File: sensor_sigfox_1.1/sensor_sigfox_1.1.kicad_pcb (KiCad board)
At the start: 2 copper layers, 27.8 x 60.1 mm, 18 parts, among them IC1 WSSFM11R2DAT, J1 Battery, J2 Conn_01x07_Socket, J3 Conn_01x01_Female, J4 Antenna, U1 ATtiny826-X, U2 MLX90393, Y1 32.768 kHz

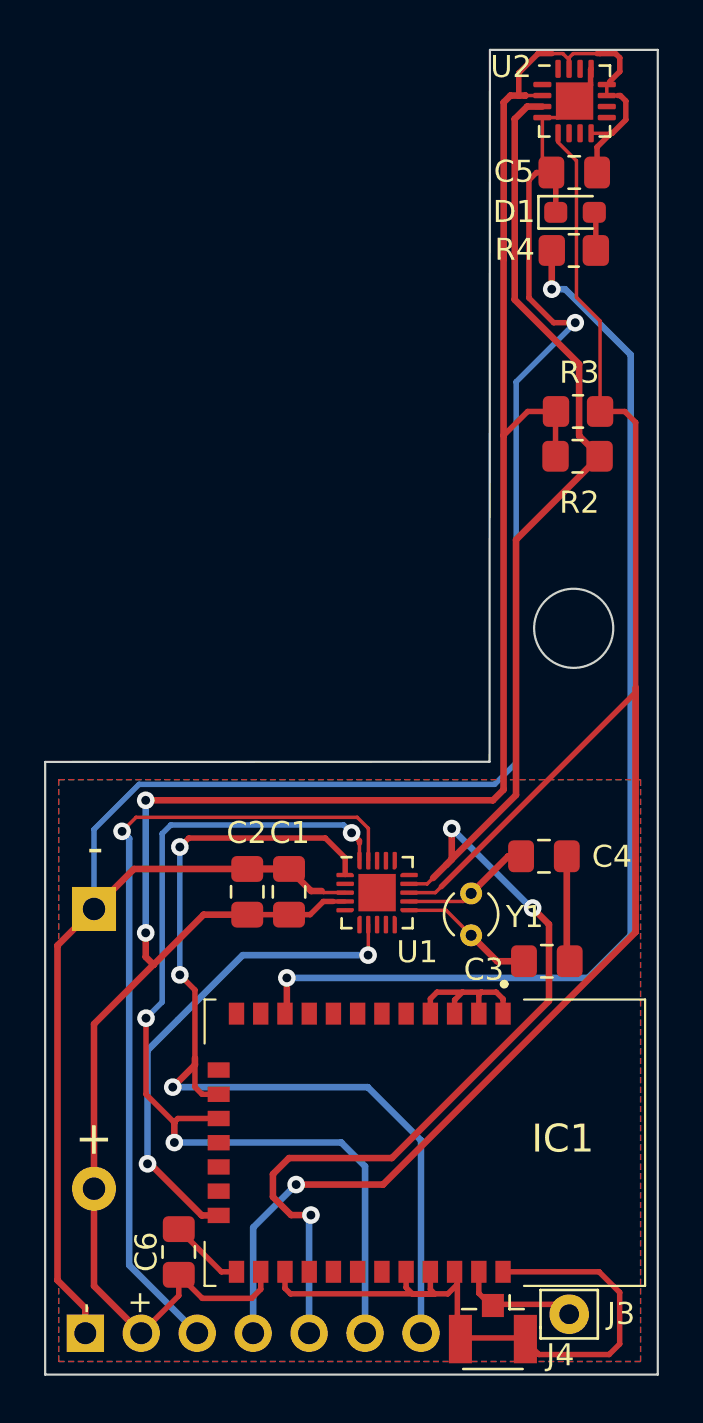
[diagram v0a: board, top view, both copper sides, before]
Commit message: pcb 1.1
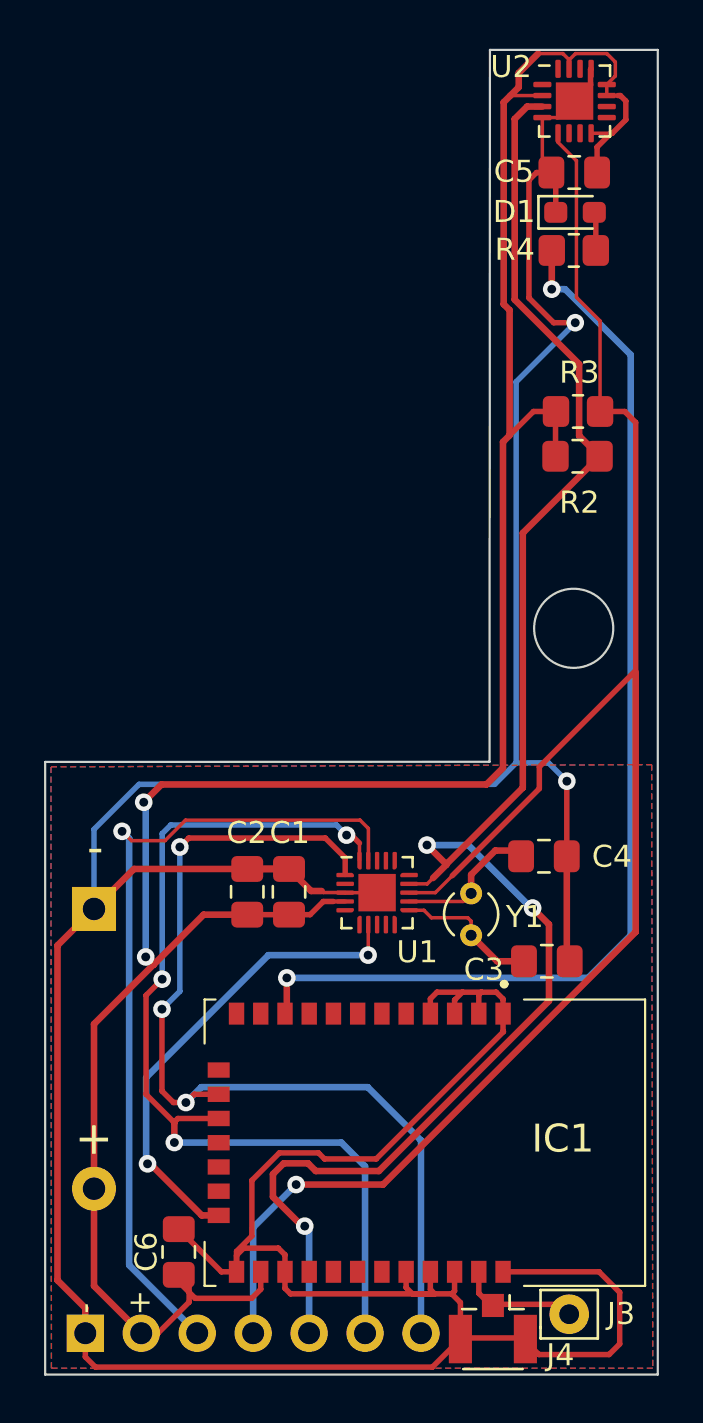
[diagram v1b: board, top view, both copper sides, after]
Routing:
- net GND: track 147.4 -> 197.0 mm, vias 1 -> 2
- net Net-(U1-PB2): track 5.94 -> 6.65 mm
- net VCC: track 114.7 -> 114.1 mm
- net Net-(IC1-RST_N): track 22.6 -> 22.0 mm

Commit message: gerber y conexiones int/trig
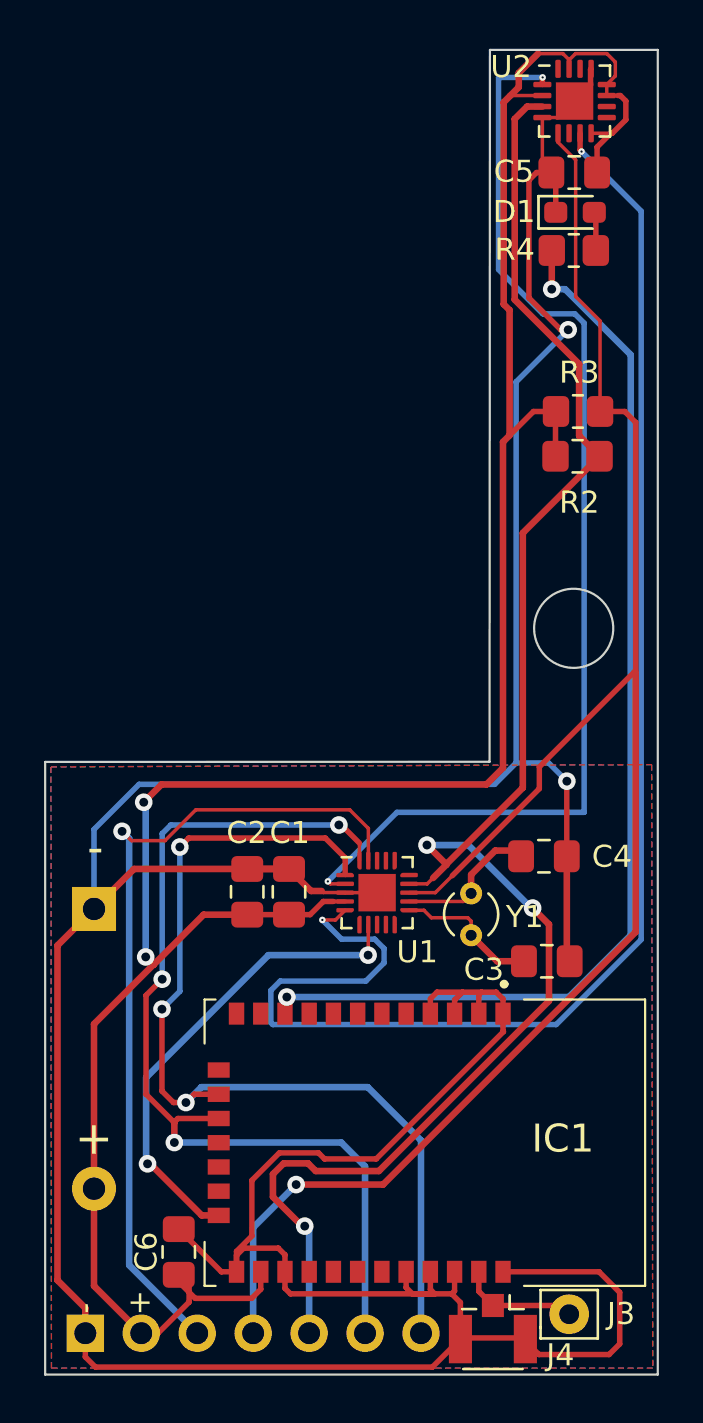
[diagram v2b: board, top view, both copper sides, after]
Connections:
- U1 pad 2: unconnected-(U1-PA3-Pad2) -> Net-(U1-PA3)
- U1 pad 5: unconnected-(U1-PA4-Pad5) -> Net-(U1-PA4)
- U2 pad 1: unconnected-(U2-INT-Pad1) -> Net-(U1-PA3)
- U2 pad 4: GND -> unconnected-(U2-N/C-Pad4)
- U2 pad 7: unconnected-(U2-INT/TRIG-Pad7) -> Net-(U1-PA4)
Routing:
- net Net-(U1-PA4): track 0.00 -> 68.5 mm, vias 0 -> 2
- net Net-(U1-PA3): track 0.00 -> 51.9 mm, vias 0 -> 2
- net GND: track 197.0 -> 196.4 mm
- net Net-(IC1-GPIO4): track 51.0 -> 50.5 mm
